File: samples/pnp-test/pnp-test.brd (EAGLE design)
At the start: 76.2 x 76.2 mm, 38 parts

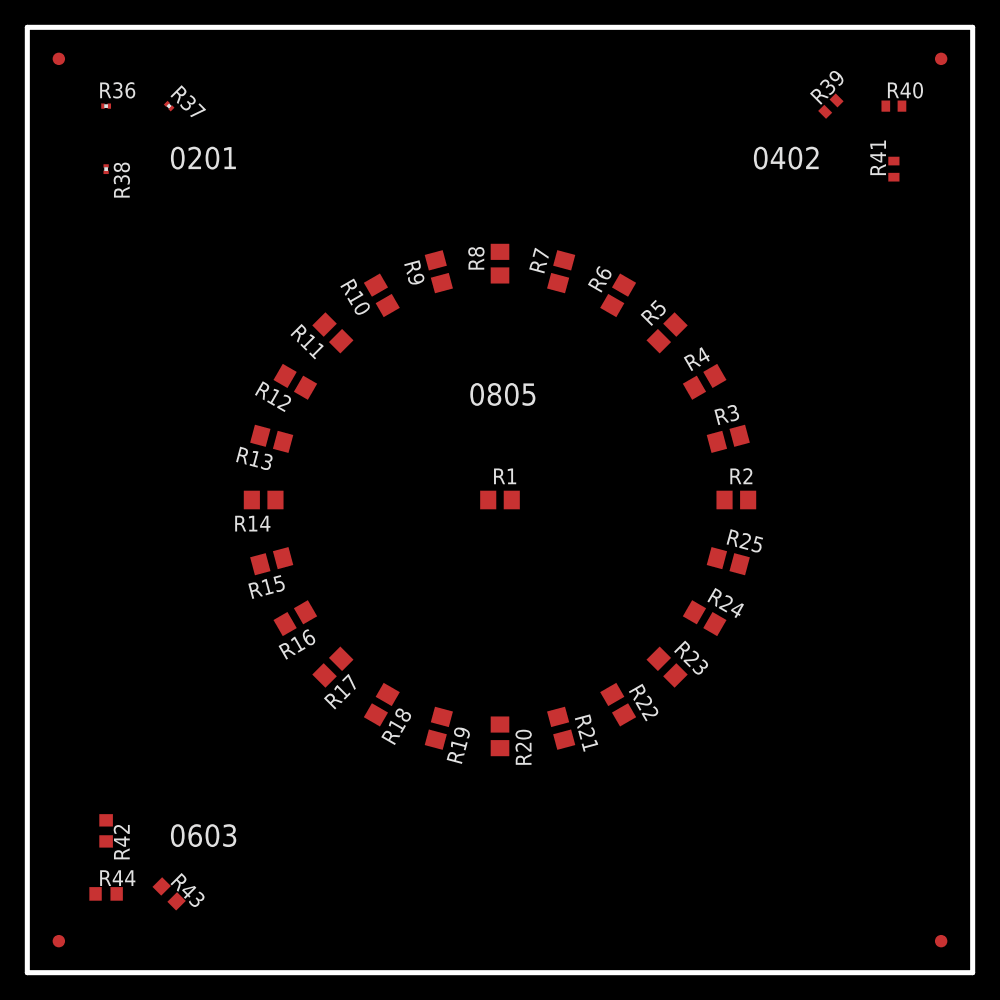
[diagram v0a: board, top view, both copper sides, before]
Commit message: Put together a full demo suite. Fresh install now boots clean and can immediately run the pnp-test job.
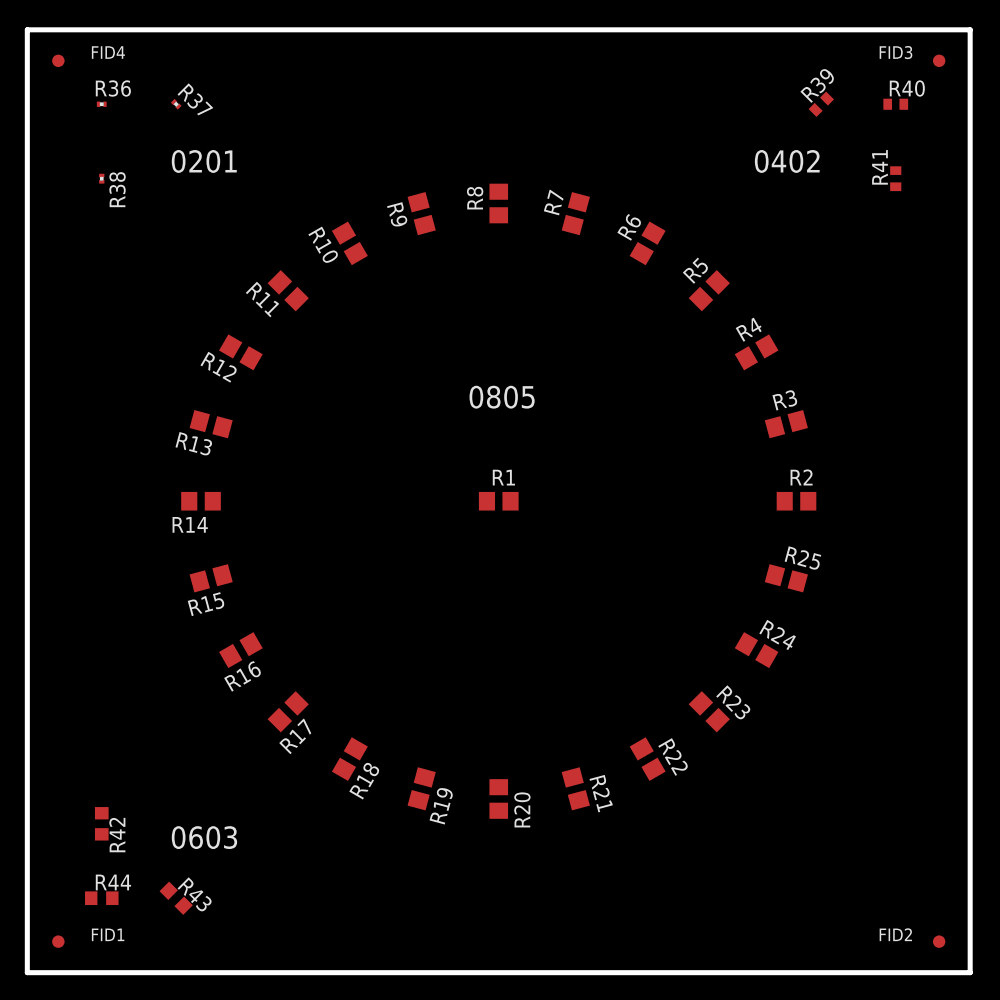
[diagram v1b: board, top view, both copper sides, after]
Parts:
- removed U$1, U$2, U$3, U$4: FIDUCIAL1X2, SparkFun:FIDUCIAL-1X2
- added FID1, FID2, FID3, FID4: FIDUCIAL1X2, SparkFun:FIDUCIAL-1X2
- R1, R10, R11, R12, R13, R14, R15, R16, R17, R18, R19, R2, R20, R21, R22, R23, R24, R25, R3, R36, R37, R38, R39, R4, R40, R41, R42, R43, R44, R5, R6, R7, R8, R9: value (none) -> 1K
- moved R17 5.09 mm to (21.0, 21.0)
- moved R16 5.09 mm to (17.2, 26.0)
- moved R18 5.09 mm to (26.0, 17.2)
- moved R15 5.07 mm to (14.8, 31.8)
- moved R19 5.07 mm to (31.8, 14.8)
- moved R14 5.05 mm to (14.0, 38.0)
- moved R20 5.05 mm to (38.0, 14.0)
- moved R13 5.02 mm to (14.8, 44.2)
- moved R21 5.02 mm to (44.2, 14.8)
- moved R12 4.99 mm to (17.2, 50.0)
- moved R22 4.99 mm to (50.0, 17.2)
- moved R11 4.95 mm to (21.0, 55.0)
- moved R23 4.95 mm to (55.0, 21.0)
- moved R10 4.92 mm to (26.0, 58.8)
- moved R24 4.92 mm to (58.8, 26.0)
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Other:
- board size 76.2 x 76.2 mm -> 76 x 76 mm
- board text added: "FID1"
- board text added: "FID2"
- board text added: "FID3"
- board text added: "FID4"
